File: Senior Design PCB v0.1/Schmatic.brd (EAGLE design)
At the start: 90.2 x 65.7 mm, 233 parts, among them IC1 TMC2208, IC2 TMC2208, IC3 TMC2208, IC4 TMC2208, IC5 TMC2208, IC6 CP2104, Q1 mmbt2222, Q2 mmbt2222, Q3 MMBT4403, Q4 AOD417, Q5 MMBT4403, Q6 MMBT4403, Q7 DMG3415U, U1 PCA9685, U2 AP2112-3.3, U3 HTU21DF, U4 HX711, U5 HX711, U6 HX711, X2 ESP32_WROOM32_SKINNY

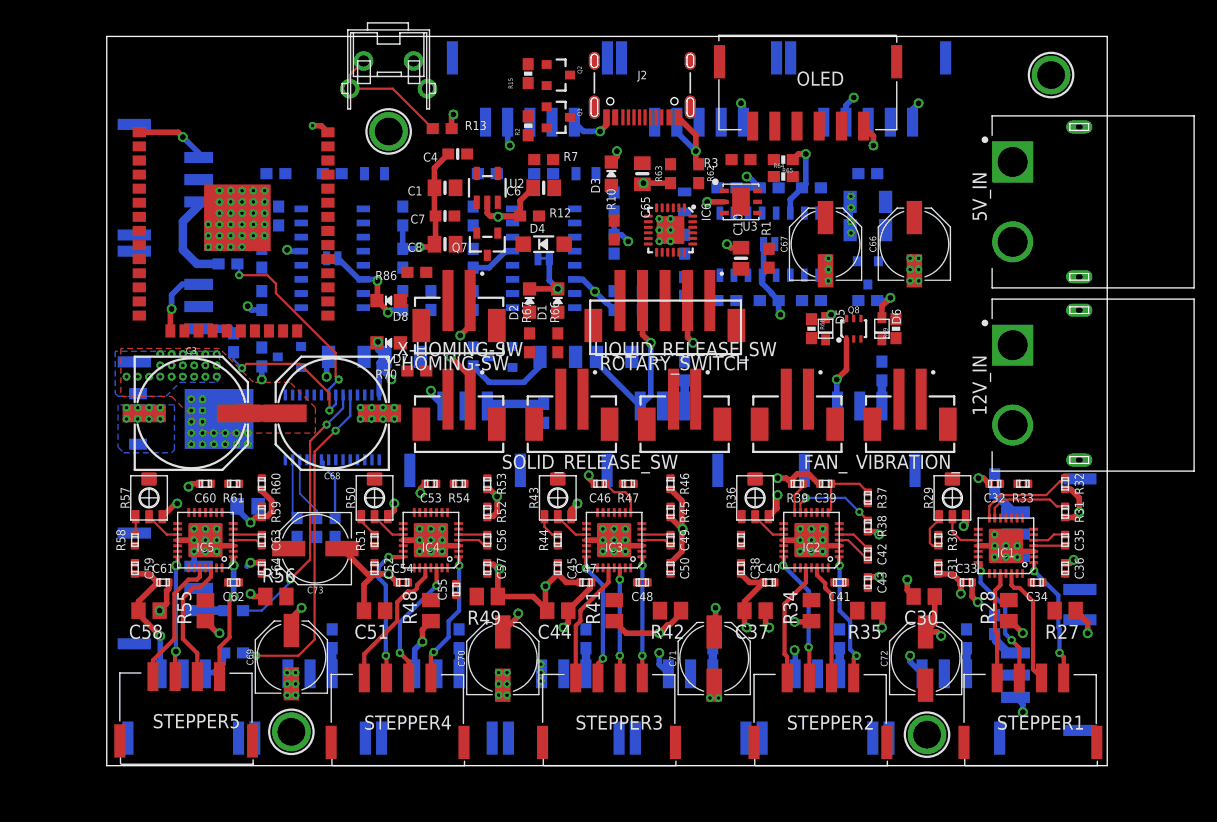
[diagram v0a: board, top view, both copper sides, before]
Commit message: done all routing
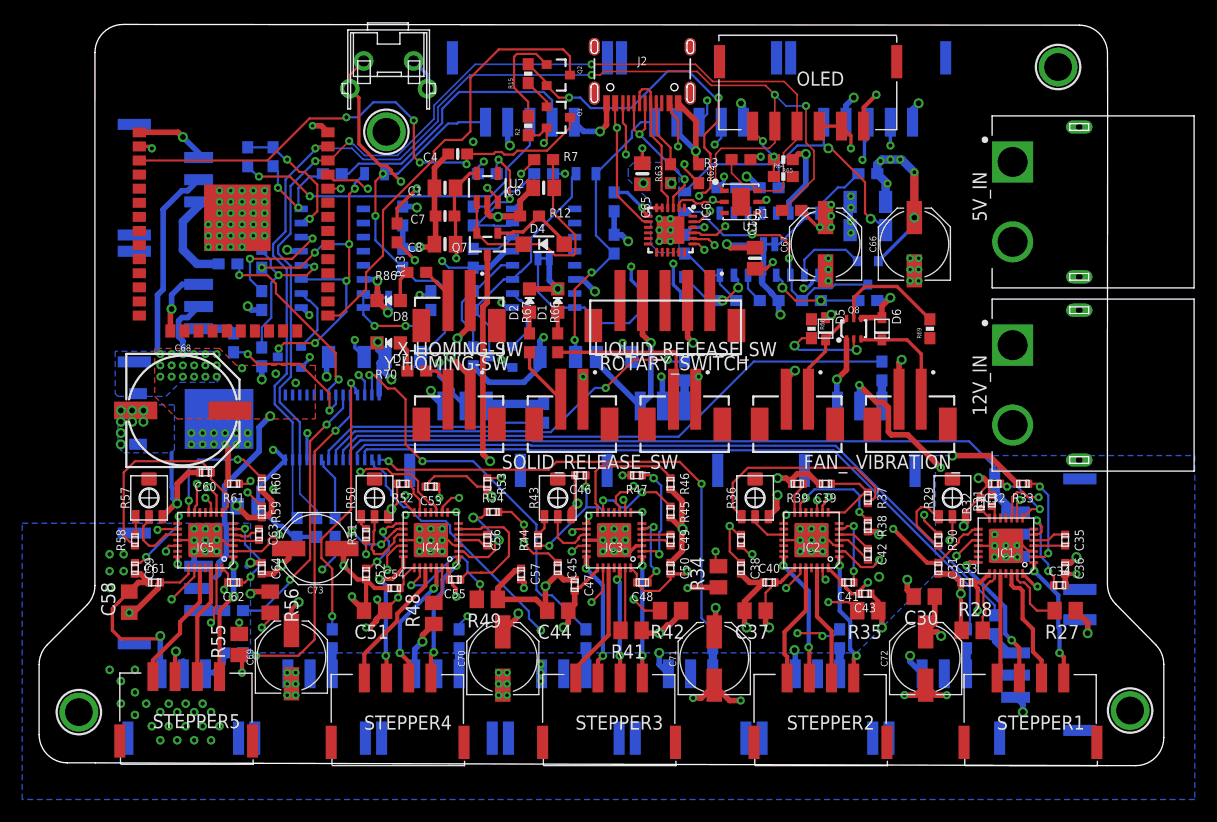
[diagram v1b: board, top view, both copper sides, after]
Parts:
- removed C15, C22, C29: 0.1uF, SparkFun-Capacitors:0603-CAP
- removed C3: 560uF, SparkFun-Capacitors:PANASONIC_G
- removed D3: RED, microbuilder:CHIPLED_0805_NOOUTLINE
- removed R10: 1K, microbuilder:0603-NO@1
- moved U$4 19.2 mm to (-2.51, 4.82)
- moved U$48 18.4 mm to (92.2, 4.97)
- moved C68 13.5 mm to (6.86, 32.0), turned to 0 degrees
- moved R13 10.2 mm to (26.2, 48.0), turned to 270 degrees
- moved R34 8.92 mm to (55.1, 17.0)
- moved R52 8.03 mm to (26.7, 25.4), turned to 90 degrees
- moved R32 7.82 mm to (78.7, 23.6), turned to 0 degrees
- moved R31 6.68 mm to (79.8, 23.9), turned to 0 degrees
- moved SJ3 5.79 mm to (24.9, 42.2)
- moved C25 5.36 mm to (15.0, 54.9), turned to 270 degrees
- moved R1 4.77 mm to (61.7, 50.0), turned to 180 degrees
- moved R55 4.31 mm to (11.9, 10.9)
- moved R54 3.97 mm to (34.8, 22.9), turned to 270 degrees
- moved R28 3.75 mm to (78.0, 12.2), turned to 0 degrees
- moved C57 3.09 mm to (37.3, 17.3)
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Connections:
- net EN_3 renamed EN_LIQUID_1
- net EN_4 renamed EN_LIQUID_3
- net EN_5 renamed EN_LIQUID_2
- removed net DIR_3: IC3.19
- removed net DIR_4: IC4.19
- removed net DIR_5: IC5.19
- removed net EN_1: IC1.2, R33.2
- removed net EN_2: IC2.2, R40.2
- removed net MS1_1: IC1.9
- removed net MS1_2: IC2.9
- removed net MS1_3: IC3.9
- removed net MS1_4: IC4.9
- removed net MS1_5: IC5.9
- removed net MS2_1: IC1.10
- removed net MS2_2: IC2.10
- removed net MS2_3: IC3.10
- removed net MS2_4: IC4.10
- removed net MS2_5: IC5.10
- removed net N$5: D3.A, R10.2
- removed net STEP_3: IC3.16
- removed net STEP_4: IC4.16
- removed net STEP_5: IC5.16
- removed net VDD: C15.1, C22.1, C29.1
- new net DIR_LIQUID: IC3.19, IC4.19, IC5.19
- new net EN_XY: IC1.2, IC2.2, R33.2, R40.2
- new net MS1_LIQUID: IC3.9, IC4.9, IC5.9
- new net MS1_SOLID: IC1.9, IC2.9
- new net MS2_LIQUID: IC3.10, IC4.10, IC5.10
- new net MS2_SOLID: IC1.10, IC2.10
- new net STEP_LIQUID: IC3.16, IC4.16, IC5.16
- net 5V_SERVO: no longer C3.+
- net GND: no longer C15.2, C22.2, C29.2, C3.-, D3.C
- net ONBOARD_LED: no longer R10.1
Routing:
- net 5V_SERVO: track 4.20 -> 115.3 mm, vias 21 -> 53
- net SDA: track 5.41 -> 112.4 mm, vias 0 -> 4
- net SCL: track 5.88 -> 101.3 mm, vias 0 -> 3
- net VCC: track 9.40 -> 102.6 mm, vias 3 -> 36
- net 5V_REG: track 0.00 -> 89.7 mm, vias 18 -> 27
- net N$39: track 0.00 -> 65.3 mm
- net GND: track 321.4 -> 386.3 mm, vias 199 -> 193
- net N$40: track 0.00 -> 64.5 mm
- net N$38: track 0.00 -> 60.9 mm
- net MS2_LIQUID: track 0.00 -> 55.5 mm, vias 0 -> 4
- net N$50: track 0.00 -> 52.8 mm
- net RXD0: track 0.00 -> 52.0 mm, vias 0 -> 2
- net N$41: track 0.00 -> 51.9 mm, vias 0 -> 3
- net 12V_REG: track 23.6 -> 74.1 mm, vias 8 -> 19
- net MS1_LIQUID: track 0.00 -> 49.8 mm, vias 0 -> 3
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- added copper zone on layer 2, net 5V_SERVO
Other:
- board size 90.2 x 65.7 mm -> 101.3 x 66.8 mm
